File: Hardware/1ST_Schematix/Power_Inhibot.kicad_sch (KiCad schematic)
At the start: 27 parts, among them J1 USB_C_Receptacle_USB2.0_16P, U2 BQ25896RTW, U3 LP2985-3.3, U4 USBLC6-2SC6

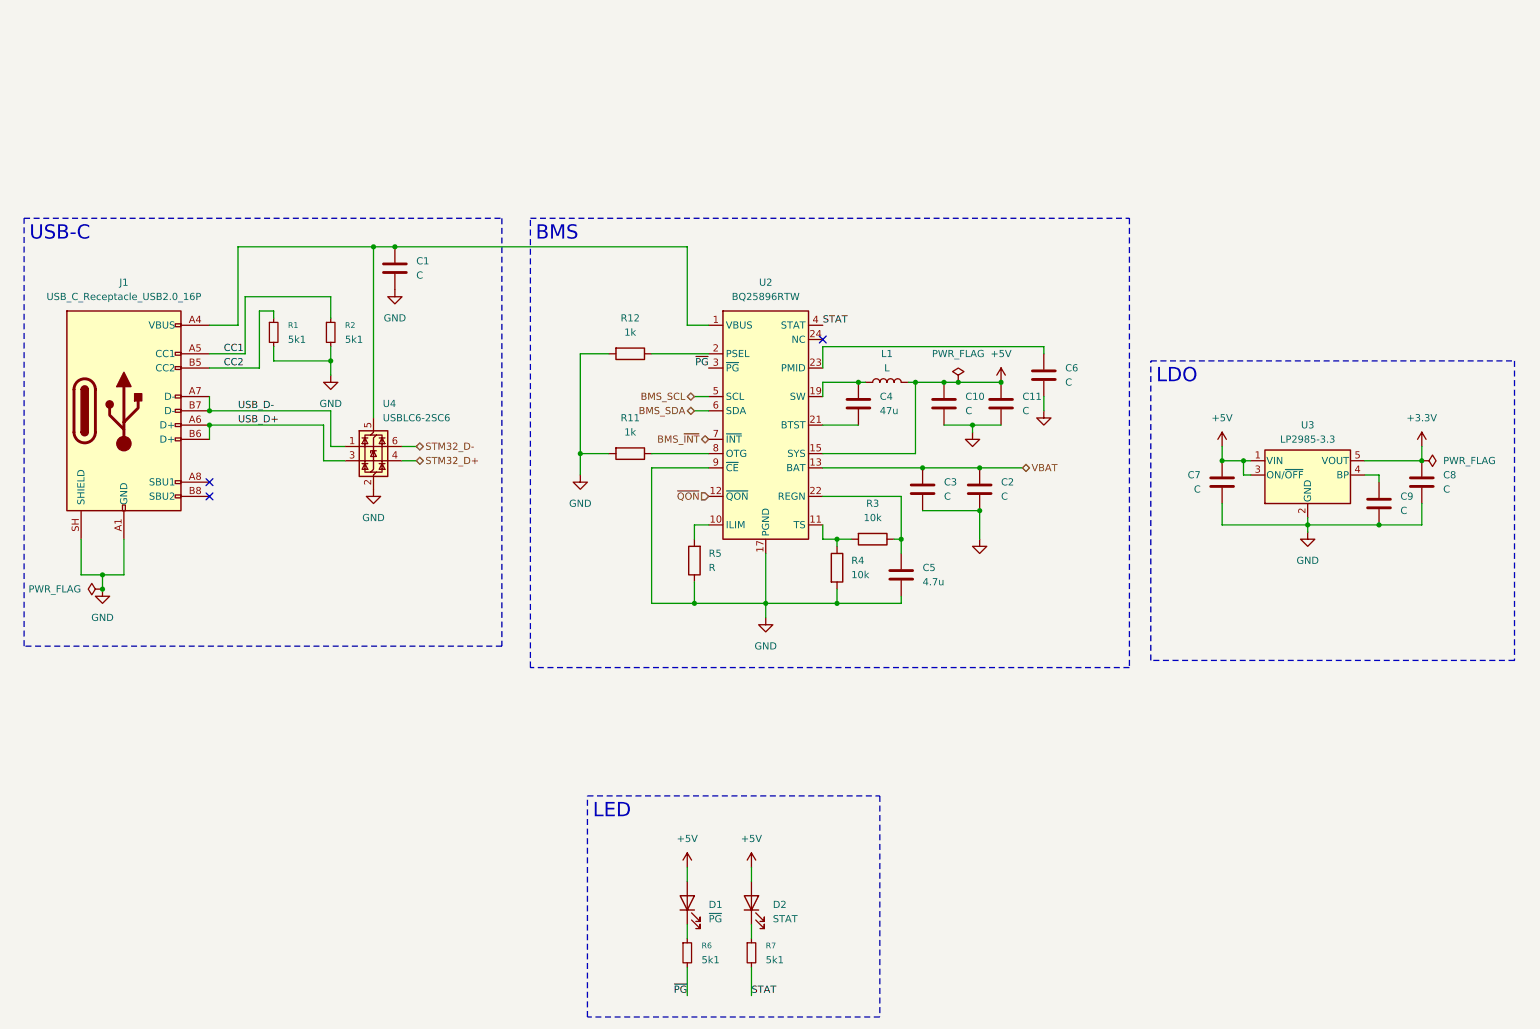
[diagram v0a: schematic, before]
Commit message: Update KiCad + Création Soft_Inhibot.ioc
Soft_Inhibot est mieux que juste Software. C'est mon avis...
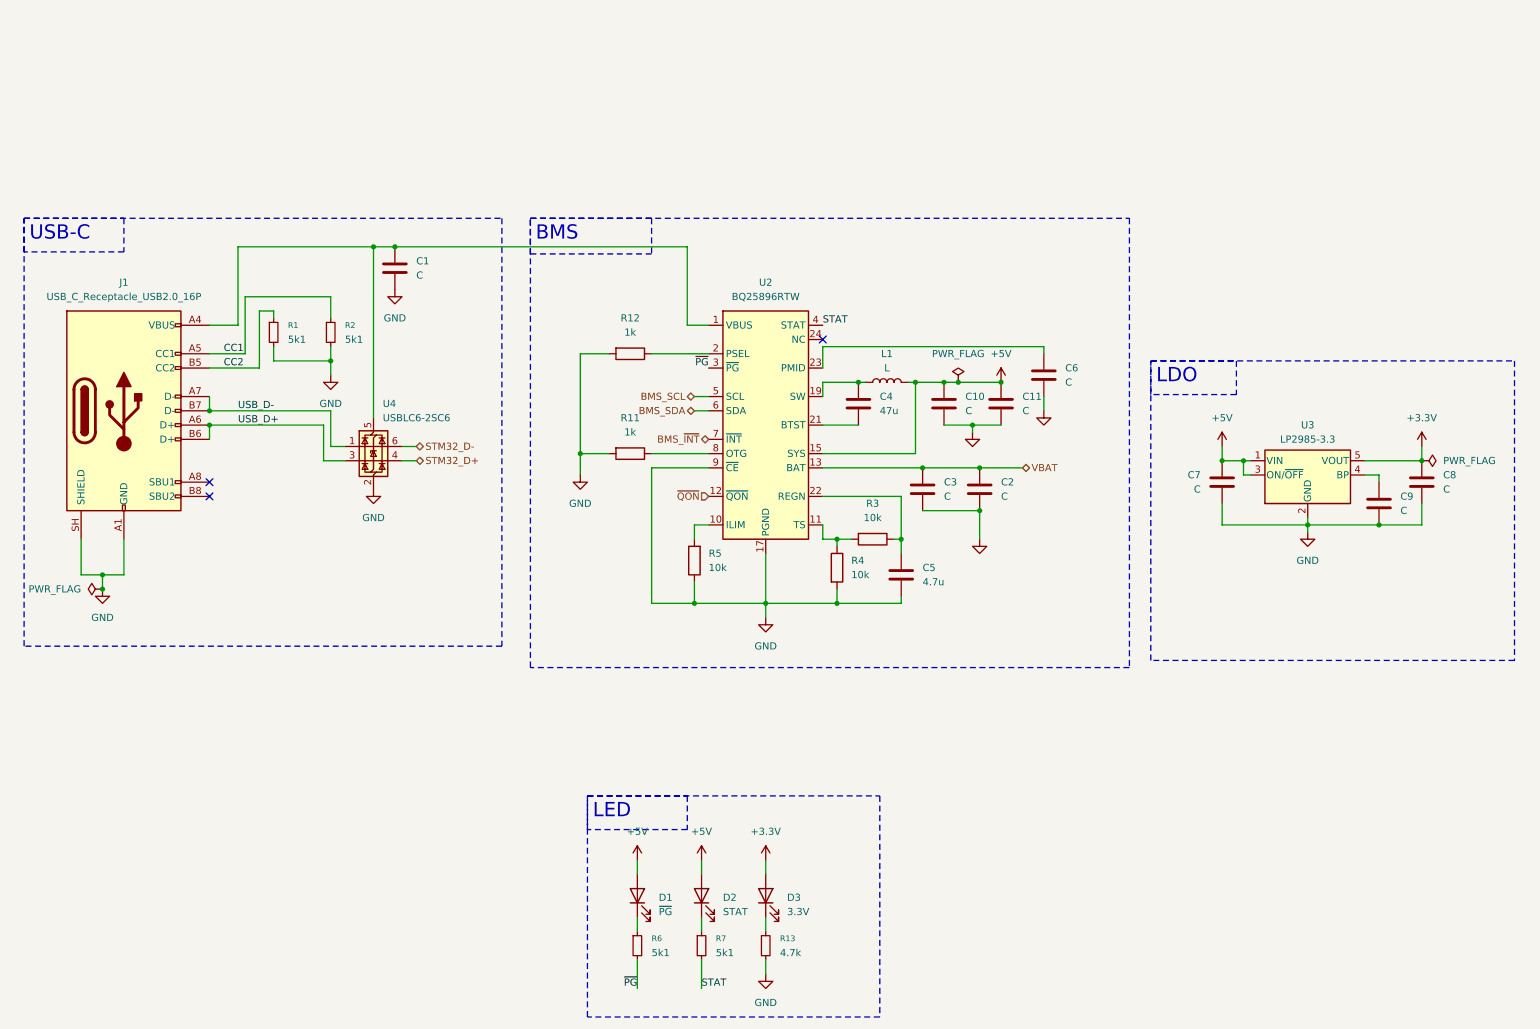
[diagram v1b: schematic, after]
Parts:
- added D3: 3.3V, Package_DFN_QFN:Texas_RTW_WQFN-24-1EP_4x4mm_P0.5mm_EP2.7x2.7mm_ThermalVias, symbol Device:LED
- added R13: 4.7k, Resistor_SMD:R_0402_1005Metric, symbol Device:R_Small
- R5: value R -> 10k
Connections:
- net +3.3V: now also D3.2 (A)
- net GND: now also R13.2
- new net: D3.1 (K), R13.1
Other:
- title: (none) -> Inhibot
- moved on the sheet: D1, D2, R6, R7

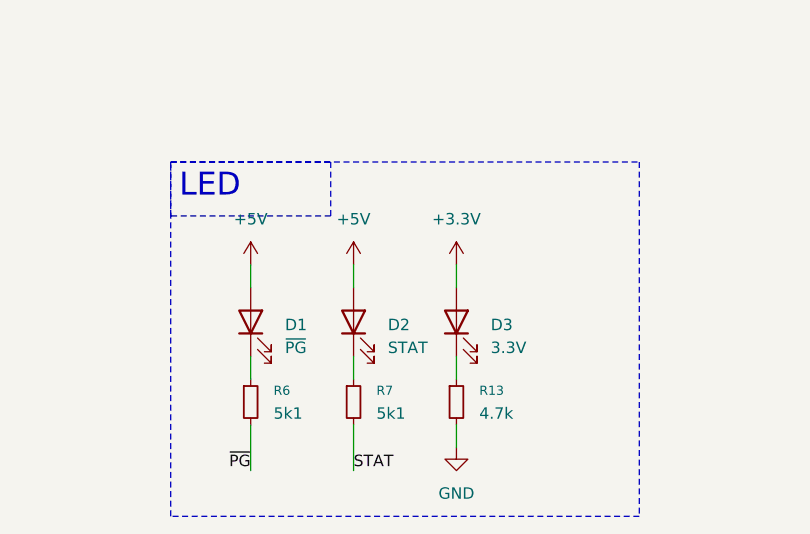
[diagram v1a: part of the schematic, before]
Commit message: Update PCB
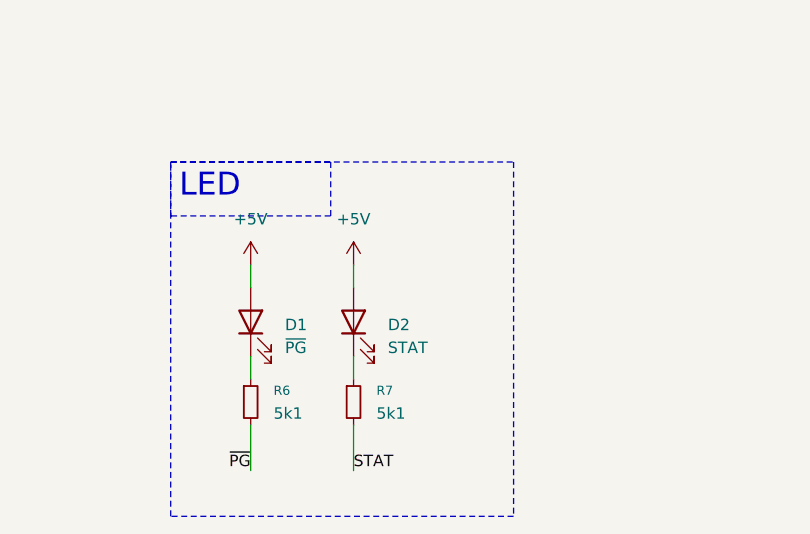
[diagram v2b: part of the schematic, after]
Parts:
- removed D3: 3.3V, Package_DFN_QFN:Texas_RTW_WQFN-24-1EP_4x4mm_P0.5mm_EP2.7x2.7mm_ThermalVias, symbol Device:LED
- removed R13: 4.7k, Resistor_SMD:R_0402_1005Metric, symbol Device:R_Small

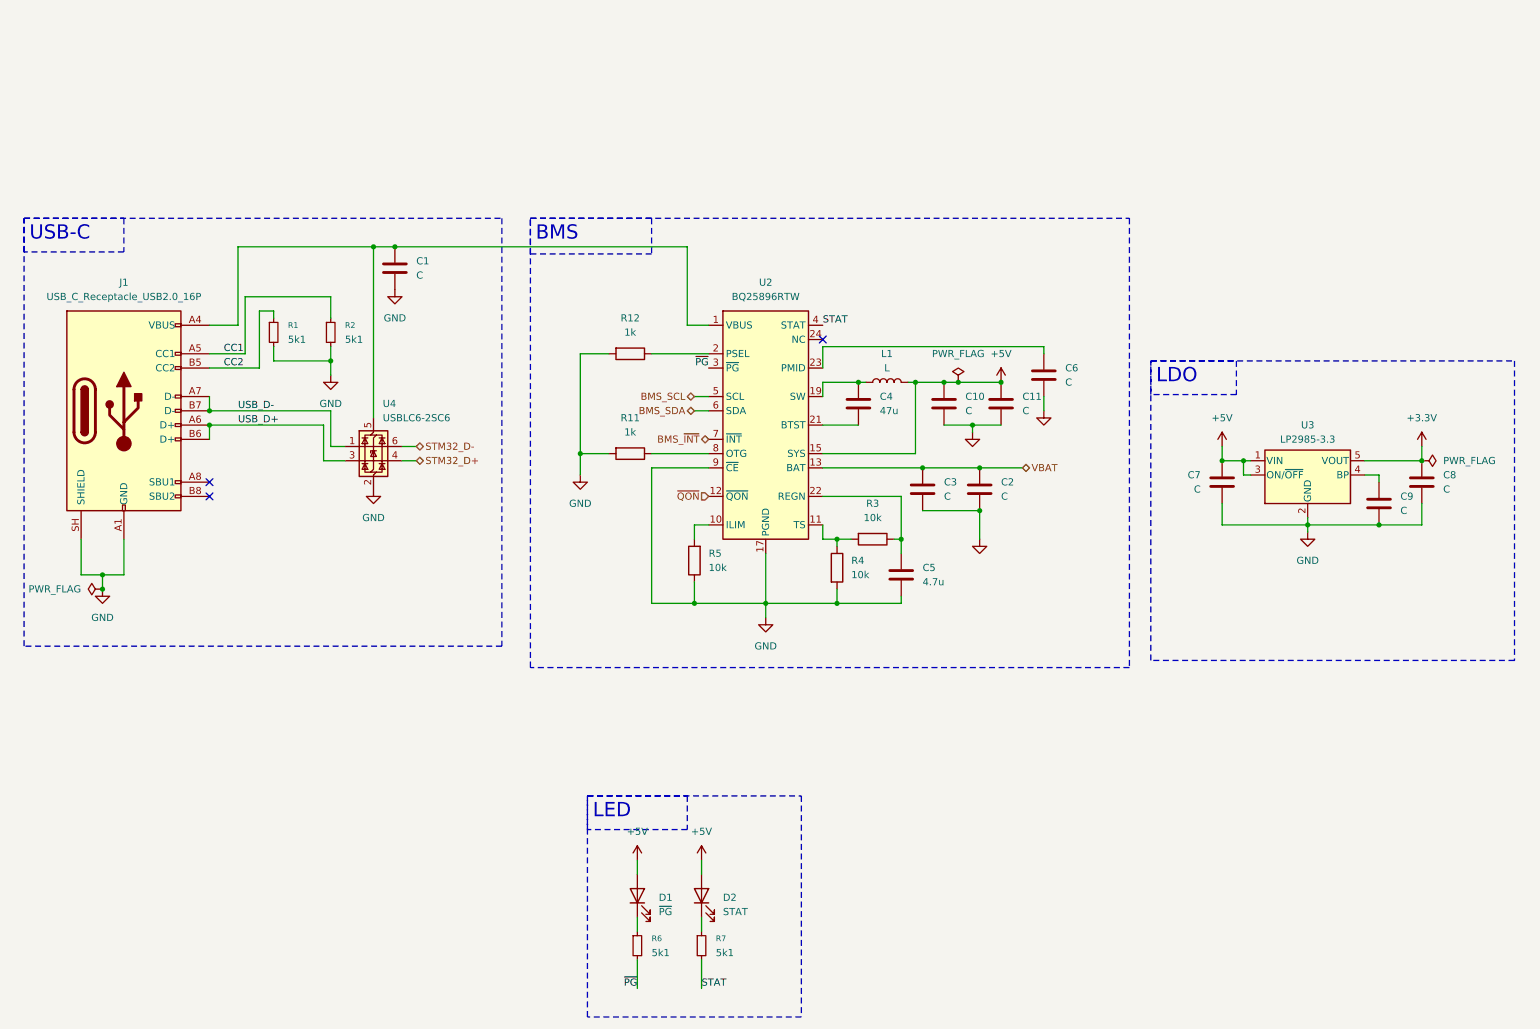
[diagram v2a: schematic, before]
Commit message: Power Update Kicad
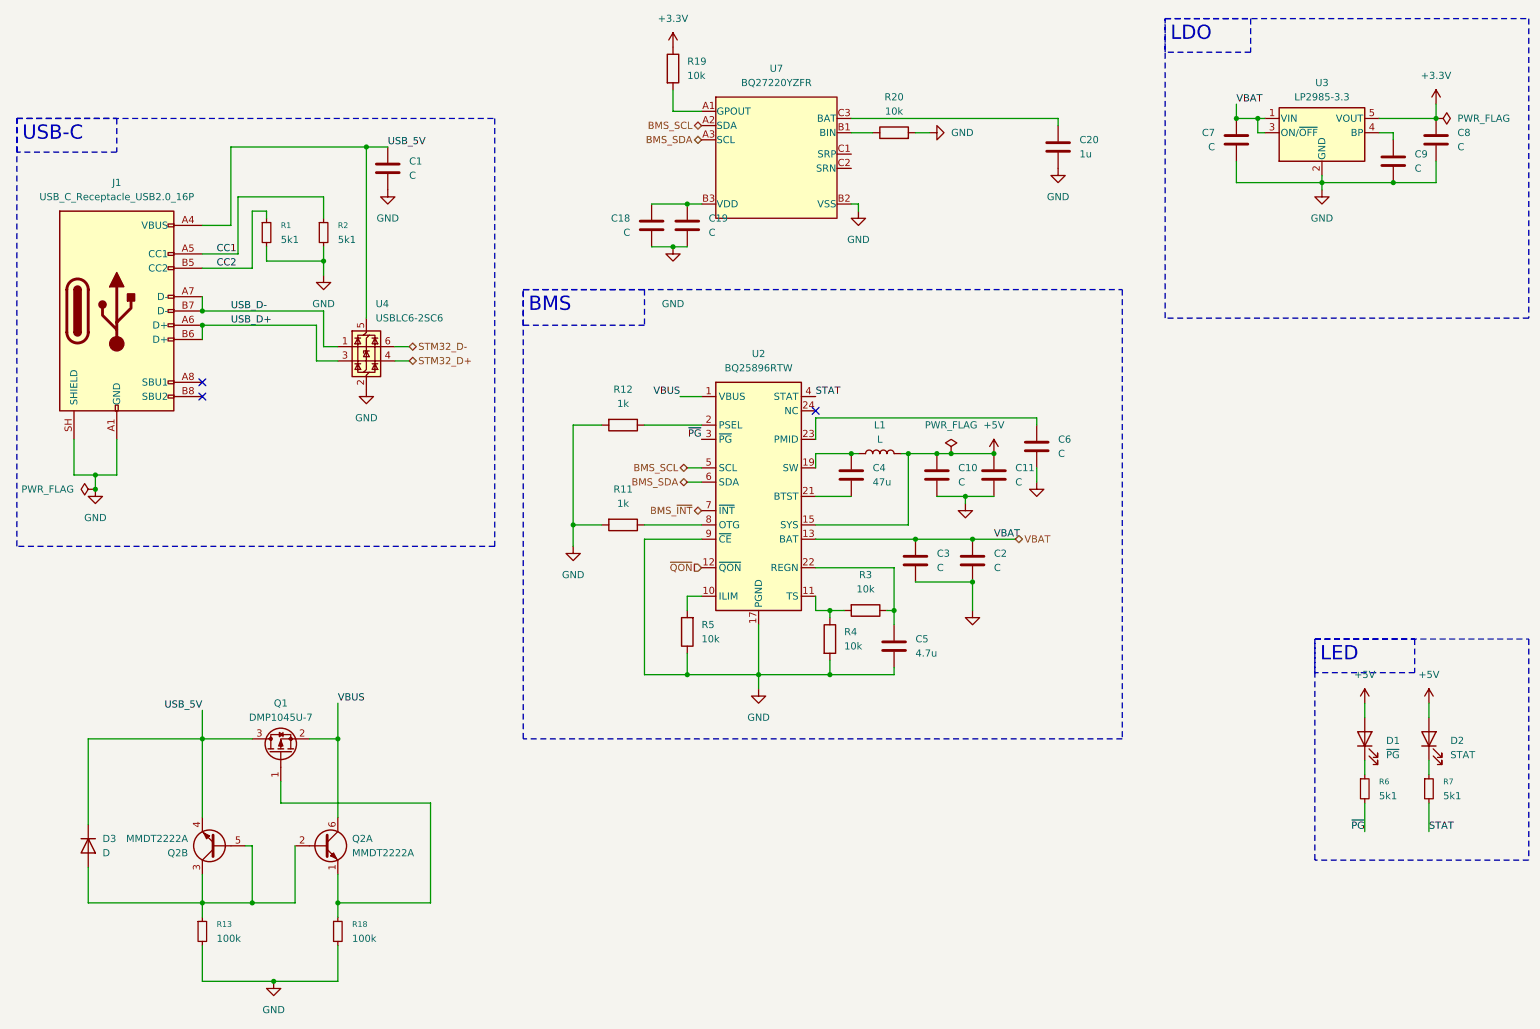
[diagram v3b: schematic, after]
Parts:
- added C18, C19: C, symbol Device:C
- added C20: 1u, symbol Device:C
- added D3: D, Diode_THT:Diode_Bridge_IXYS_GUFP, symbol Device:D
- added Q1: DMP1045U-7, Package_TO_SOT_SMD:SOT-23, symbol Transistor_FET:DMP3099L
- added Q2: MMDT2222A, Package_TO_SOT_SMD:SOT-363_SC-70-6, symbol Transistor_BJT:MMDT2222A
- added R13, R18: 100k, Package_TO_SOT_SMD:SOT-363_SC-70-6, symbol Device:R_Small
- added R19, R20: 10k, symbol Device:R
- added U7: BQ27220YZFR, Package_BGA:Texas_DSBGA-9_1.4715x1.4715mm_Layout3x3_P0.5mm, symbol inhibot_lib:BQ27220YZFR
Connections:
- net +3.3V: now also R19.1
- net +5V: no longer C7.1, U3.1 (VIN), U3.3 (ON/~{OFF})
- net BMS_SCL: now also U7.A2 (SDA)
- net BMS_SDA: now also U7.A3 (SCL)
- net GND: now also C18.2, C19.2, C20.2, R13.2, R18.2, R20.2, U7.B2 (VSS)
- net VBAT: now also C7.1, U3.1 (VIN), U3.3 (ON/~{OFF})
- net USB_5V: now reaches C1.1, J1.A4 (VBUS), J1.A9 (VBUS), J1.B4 (VBUS), J1.B9 (VBUS), U4.5 (VBUS)
- net USB_5V: now also D3.1 (K), Q1.3 (D), Q2.4 (E2); no longer U2.1 (VBUS)
- new net: Q1.1 (G), Q2.1 (E1), R18.1
- new net: D3.2 (A), Q2.2 (B1), Q2.3 (C2), Q2.5 (B2), R13.1
- new net: C18.1, C19.1, U7.B3 (VDD)
- new net: R20.1, U7.B1 (BIN)
- new net: R19.2, U7.A1 (GPOUT)
- new net: C20.1, U7.C3 (BAT)
- new net VBUS: Q1.2 (S), Q2.6 (C1), U2.1 (VBUS)
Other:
- moved on the sheet: C1, C10, C11, C2, C3, C4, C5, C6, C7, C8, C9, D1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
